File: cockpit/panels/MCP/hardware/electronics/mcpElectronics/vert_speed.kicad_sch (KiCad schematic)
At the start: 1 part

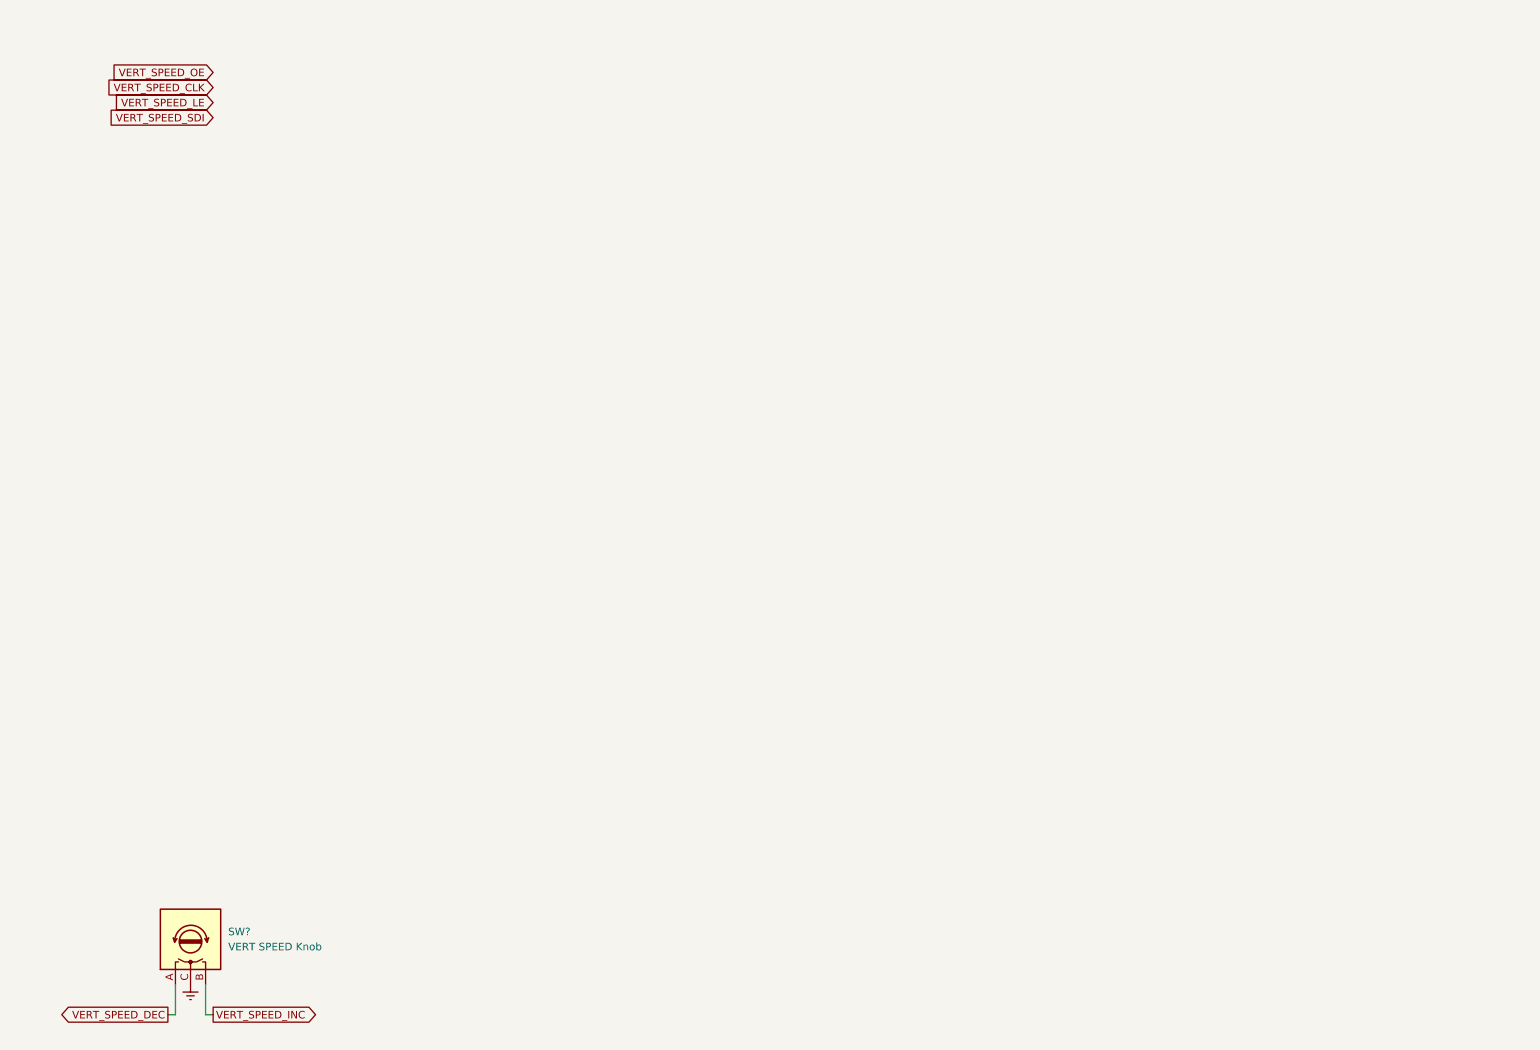
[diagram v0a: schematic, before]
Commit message: update
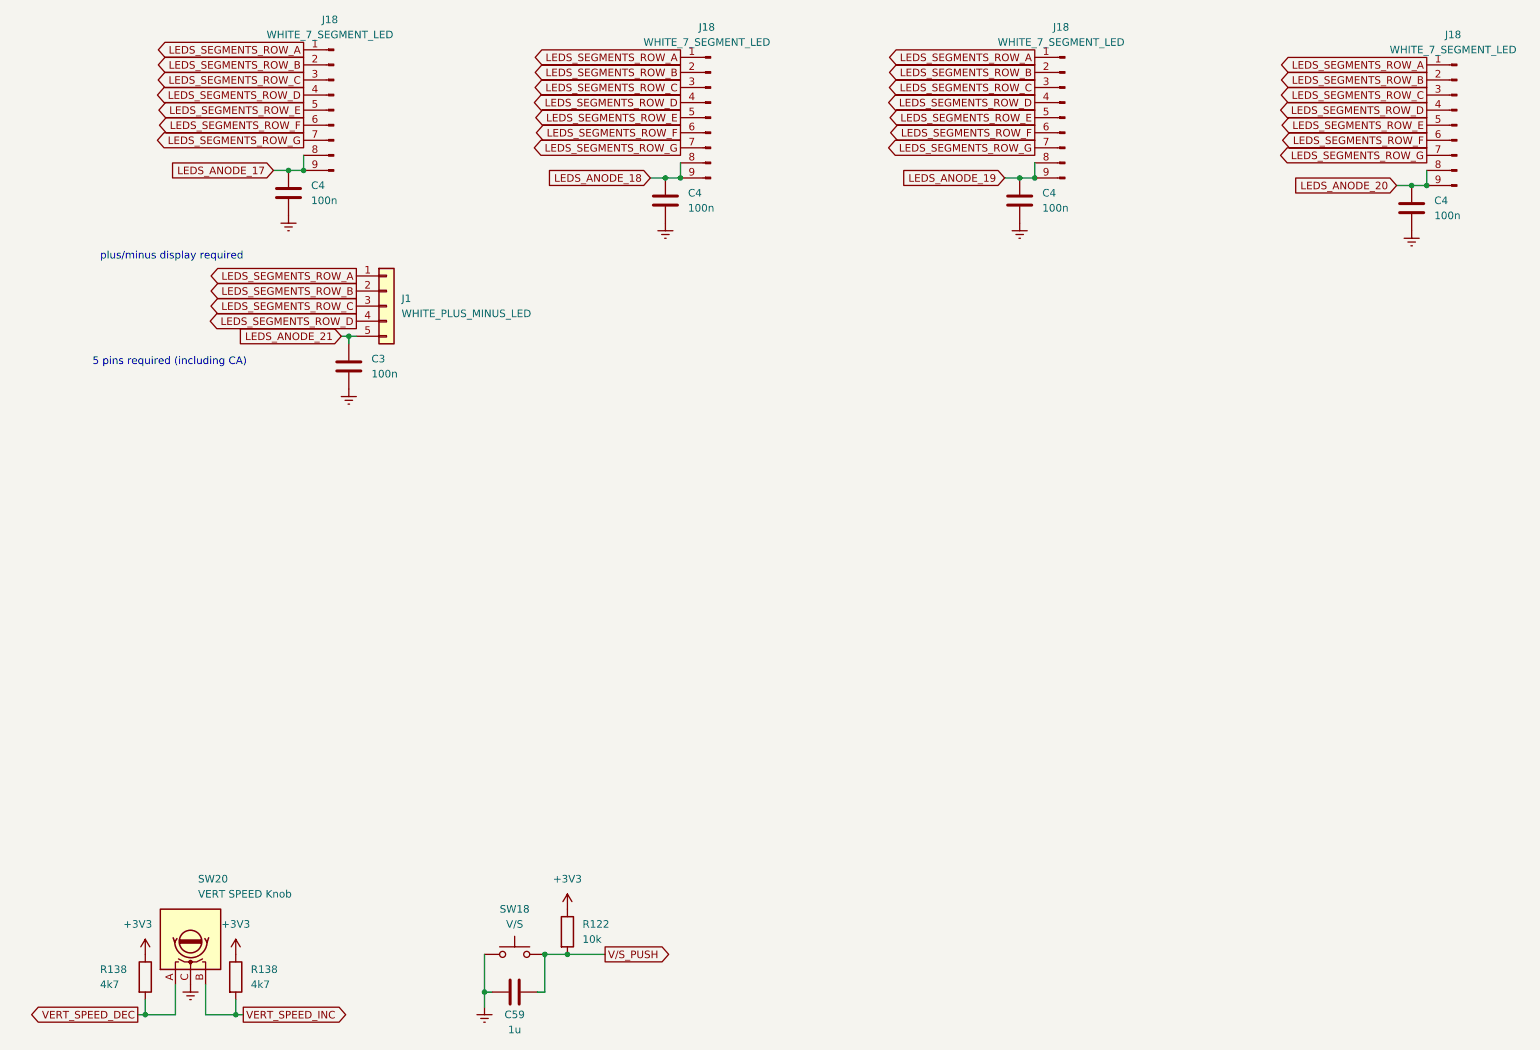
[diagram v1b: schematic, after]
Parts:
- added C3, C4 (x4): 100n, Capacitor_SMD:C_0402_1005Metric, symbol Device:C
- added C59: 1u, Capacitor_SMD:C_0402_1005Metric, symbol Device:C
- added J1: WHITE_PLUS_MINUS_LED, Connector_PinHeader_2.54mm:PinHeader_1x05_P2.54mm_Vertical, symbol Connector_Generic:Conn_01x05
- added J18 (x4): WHITE_7_SEGMENT_LED, Connector_PinHeader_2.54mm:PinHeader_1x09_P2.54mm_Vertical, symbol Connector:Conn_01x09_Pin
- added R122: 10k, Resistor_SMD:R_0402_1005Metric, symbol Device:R
- added R138 (x2): 4k7, Resistor_SMD:R_0402_1005Metric, symbol Device:R
- added SW18: V/S, Button_Switch_THT:SW_PUSH_6mm_H5mm, symbol Switch:SW_Push
- SW20: renamed from SW?; footprint (none) -> Rotary_Encoder:RotaryEncoder_Bourns_Vertical_PEC12R-3x17F-Nxxxx
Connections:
- net Earth: now also C3.2, C4.2, C4.2, C4.2, C4.2, C59.2, SW18.1
- net VERT_SPEED_DEC: now also R138.2
- net VERT_SPEED_INC: now also R138.2
- new net +3V3: R122.1, R138.1, R138.1
- new net LEDS_ANODE_17: C4.1, J18.8 (Pin_8), J18.9 (Pin_9)
- new net LEDS_ANODE_18: C4.1, J18.8 (Pin_8), J18.9 (Pin_9)
- new net LEDS_ANODE_19: C4.1, J18.8 (Pin_8), J18.9 (Pin_9)
- new net LEDS_ANODE_20: C4.1, J18.8 (Pin_8), J18.9 (Pin_9)
- new net LEDS_ANODE_21: C3.1, J1.5 (Pin_5)
- new net LEDS_SEGMENTS_ROW_A: J1.1 (Pin_1), J18.1 (Pin_1), J18.1 (Pin_1), J18.1 (Pin_1), J18.1 (Pin_1)
- new net LEDS_SEGMENTS_ROW_B: J1.2 (Pin_2), J18.2 (Pin_2), J18.2 (Pin_2), J18.2 (Pin_2), J18.2 (Pin_2)
- new net LEDS_SEGMENTS_ROW_C: J1.3 (Pin_3), J18.3 (Pin_3), J18.3 (Pin_3), J18.3 (Pin_3), J18.3 (Pin_3)
- new net LEDS_SEGMENTS_ROW_D: J1.4 (Pin_4), J18.4 (Pin_4), J18.4 (Pin_4), J18.4 (Pin_4), J18.4 (Pin_4)
- new net LEDS_SEGMENTS_ROW_E: J18.5 (Pin_5), J18.5 (Pin_5), J18.5 (Pin_5), J18.5 (Pin_5)
- new net LEDS_SEGMENTS_ROW_F: J18.6 (Pin_6), J18.6 (Pin_6), J18.6 (Pin_6), J18.6 (Pin_6)
- new net LEDS_SEGMENTS_ROW_G: J18.7 (Pin_7), J18.7 (Pin_7), J18.7 (Pin_7), J18.7 (Pin_7)
- new net V/S_PUSH: C59.1, R122.2, SW18.2
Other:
- note added: "5 pins required (including CA)"
- note added: "plus/minus display required"
